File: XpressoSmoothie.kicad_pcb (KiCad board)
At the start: 2 copper layers, 99.7 x 99.7 mm, 130 parts, among them J1 HEADER_4, J10 HEADER_3X2, J11 Pwr_in, J12 HEADER_4, J13 HEADER_4X2, J14 HEADER_3X2, J15 HEADER_4, J16 HEADER_4, J17 HEADER_4, J172 HEADER_2, J18 HEADER_4, J19 HEADER_2, J2 HEADER_4, J20 HEADER_2, J21 HEADER_2, J22 HEADER_2, J23 HEADER_4, J232 HEADER_2, J24 HEADER_4, J25 HEADER_4, J252 HEADER_2, J26 USB, J27 HEADER_4, J28 MICROSD-MOLEX, J3 HEADER_3, J4 HEADER_3X2, J5 HEADER_3X2, J6 LPCXPRESSO_GENERIC_HEADER, J7 HEADER_4, J8 HEADER_4, J9 HEADER_3X2, M1 LOGO_OSHW, M2 LOGO_OSHW, Q1 IRLB 8743, Q2 IRLB 8743, Q3 IRLB 8743, Q4 IRLB 8743, SW1 SW_PUSH, SW2 SW_PUSH, U1 POLOLU_A4988, U10 TC4422A, U11 TC4422A, U12 LM1117-3.3, U2 POLOLU_A4988, U3 POLOLU_A4988, U4 POLOLU_A4988, U5 POLOLU_A4988, U7 LM7809CT, U8 TC4422A, U9 TC4422A

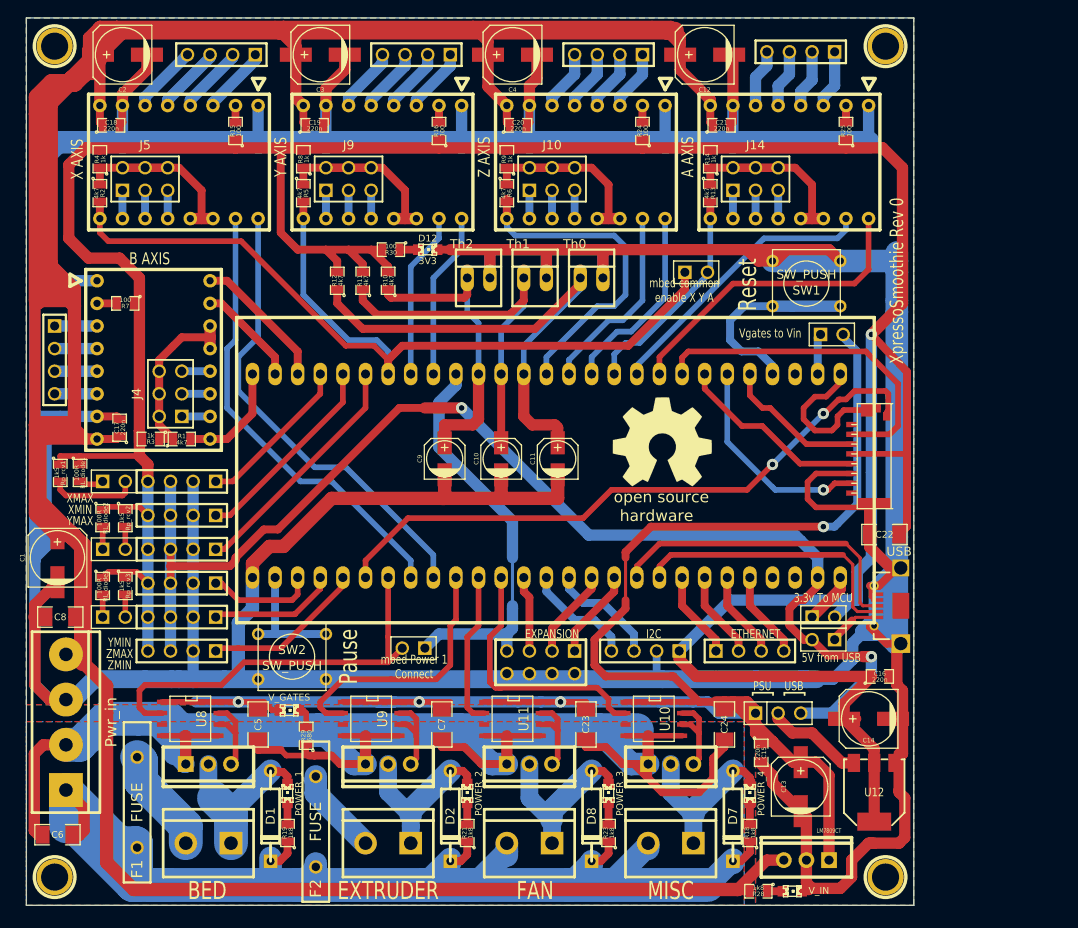
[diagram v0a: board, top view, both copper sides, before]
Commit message: Begin routing.
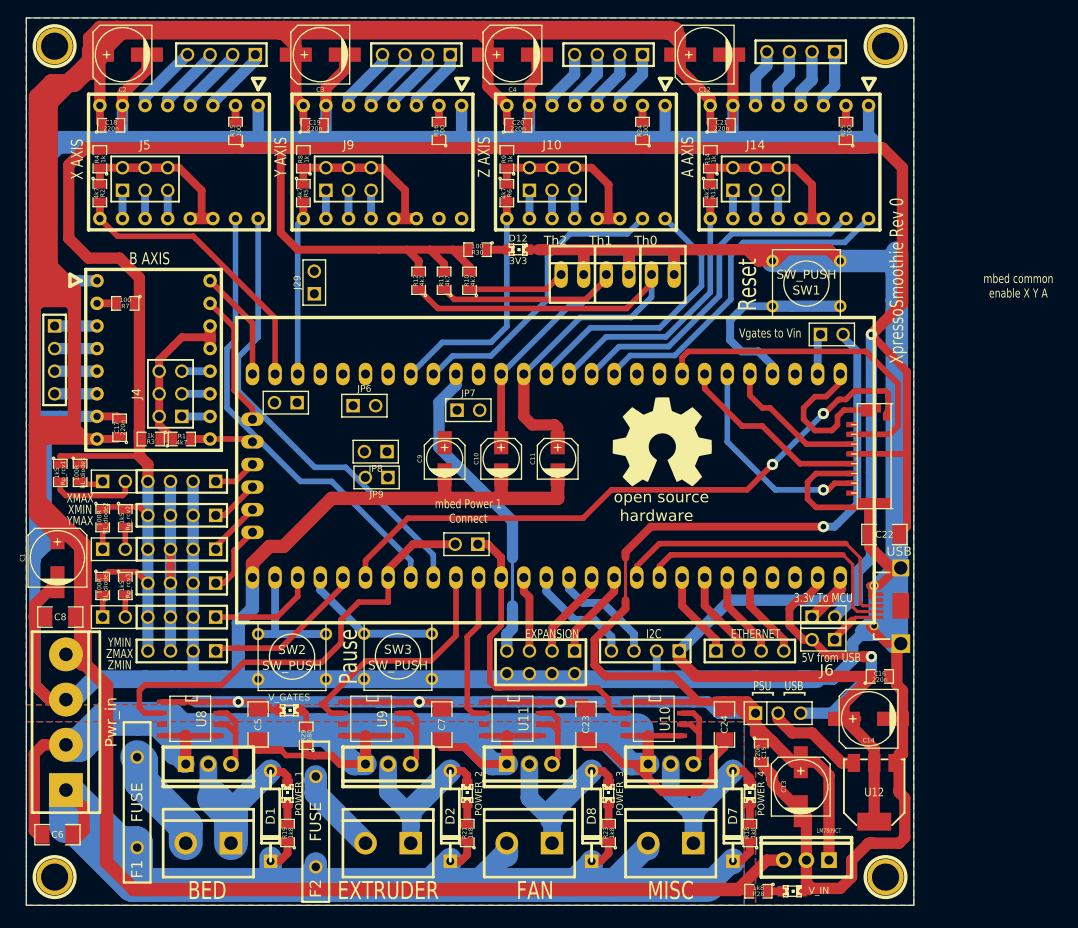
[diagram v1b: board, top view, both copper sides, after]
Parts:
- added J29: HEADER_2, PIN_ARRAY_2X1, F.Cu at (104.1, 83.7)
- added JP6: JUMPER-2, PIN_ARRAY_2X1, F.Cu at (109.7, 97.5)
- added JP7: JUMPER-2, PIN_ARRAY_2X1, F.Cu at (121.4, 98.0)
- added JP8: JUMPER-2, PIN_ARRAY_2X1, F.Cu at (111.0, 102.7)
- added JP9: JUMPER-2, PIN_ARRAY_2X1, F.Cu at (111.1, 105.6)
- added SW3: SW_PUSH, SW_PUSH_SMALL, F.Cu at (113.5, 125.7)
- J6: footprint LPCXPRESS0_GENERIC -> LPCXPRESS0_1ROW
- moved JP2 48.4 mm to (100.9, 97.2), turned to 180 degrees
- moved JP1 13.1 mm to (121.2, 113.1)
- moved Th2 10.5 mm to (133.1, 82.8)
- moved D12 10.2 mm to (127.0, 80.0)
- moved R30 9.72 mm to (122.4, 80.0)
- moved Th1 9.28 mm to (138.2, 82.8)
- moved R10 9.14 mm to (121.5, 83.5)
- moved R11 9.14 mm to (118.7, 83.5)
- moved R12 9.14 mm to (115.8, 83.5)
- moved Th0 8.01 mm to (143.3, 82.8)
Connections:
- C9 pad 1: THERM2 -> N-0000091
- J6 pad 10: A-STEP -> N-0000071
- J6 pad 11: A-EN -> A-DIR
- J6 pad 12: Z-DIR -> A-STEP
- J6 pad 13: Z-STEP -> A-EN
- J6 pad 14: Z-EN -> Z-DIR
- J6 pad 19: Y-DIR -> Z-STEP
- J6 pad 20: Y-STEP -> Z-EN
- J6 pad 21: X-EN -> N-0000073
- J6 pad 22: YMAX -> N-0000072
- J6 pad 23: XMIN -> Y-DIR
- J6 pad 24: XMAX -> Y-STEP
- J6 pad 25: B-DIR -> Y-EN
- J6 pad 26: B-STEP -> X-EN
- J6 pad 27: B-EN -> B-DIR
- J6 pad 51: ZMAX -> Bootloader
- J6 pad 52: YMIN -> ZMAX
- J6 pad 9: A-DIR -> N-0000064
- JP1 pad 1: 18_P0.26AOUT -> POWER4
- JP2 pad 1: X-EN -> Y-EN
- JP2 pad 2: A-EN -> X-EN
- R10 pad 1: THERM2 -> N-0000091
- R5 pad 2: X-EN -> Y-EN
- Th2 pad 1: THERM2 -> N-0000091
- U3 pad 9: X-EN -> Y-EN
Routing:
- net +5V: track 141.7 -> 52.3 mm, vias 2 -> 1
- net X-EN: track 108.7 -> 32.5 mm
- net THERM2: track 33.9 -> 0.00 mm
- net YMAX: track 27.2 -> 6.15 mm
- net Y-EN: track 0.00 -> 19.6 mm
- net Y-DIR: track 18.8 -> 0.00 mm
- net Y-STEP: track 18.8 -> 0.00 mm
- net XMIN: track 22.7 -> 5.44 mm
- net Bootloader: track 0.00 -> 16.0 mm
- net GND: track 762.1 -> 747.3 mm
- net XMAX: track 18.0 -> 4.92 mm
- net Z-STEP: track 21.8 -> 33.6 mm
- net N-0000091: track 0.00 -> 11.0 mm
- net 18_P0.26AOUT: track 45.5 -> 35.6 mm
- net Z-EN: track 36.5 -> 27.4 mm
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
